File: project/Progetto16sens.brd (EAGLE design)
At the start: 228.6 x 231.1 mm, 148 parts, among them IC1 LMZ14202TZE-ADJ_NOPB, J2 455-1750-1-ND, M1 43650-0201, M2 43650-0201, M3 43650-0201, M4 43650-0201, M5 ARDUINO-PRO-MINI, SW1 TL32PO, SW2 TL32PO, SW3 TL32PO

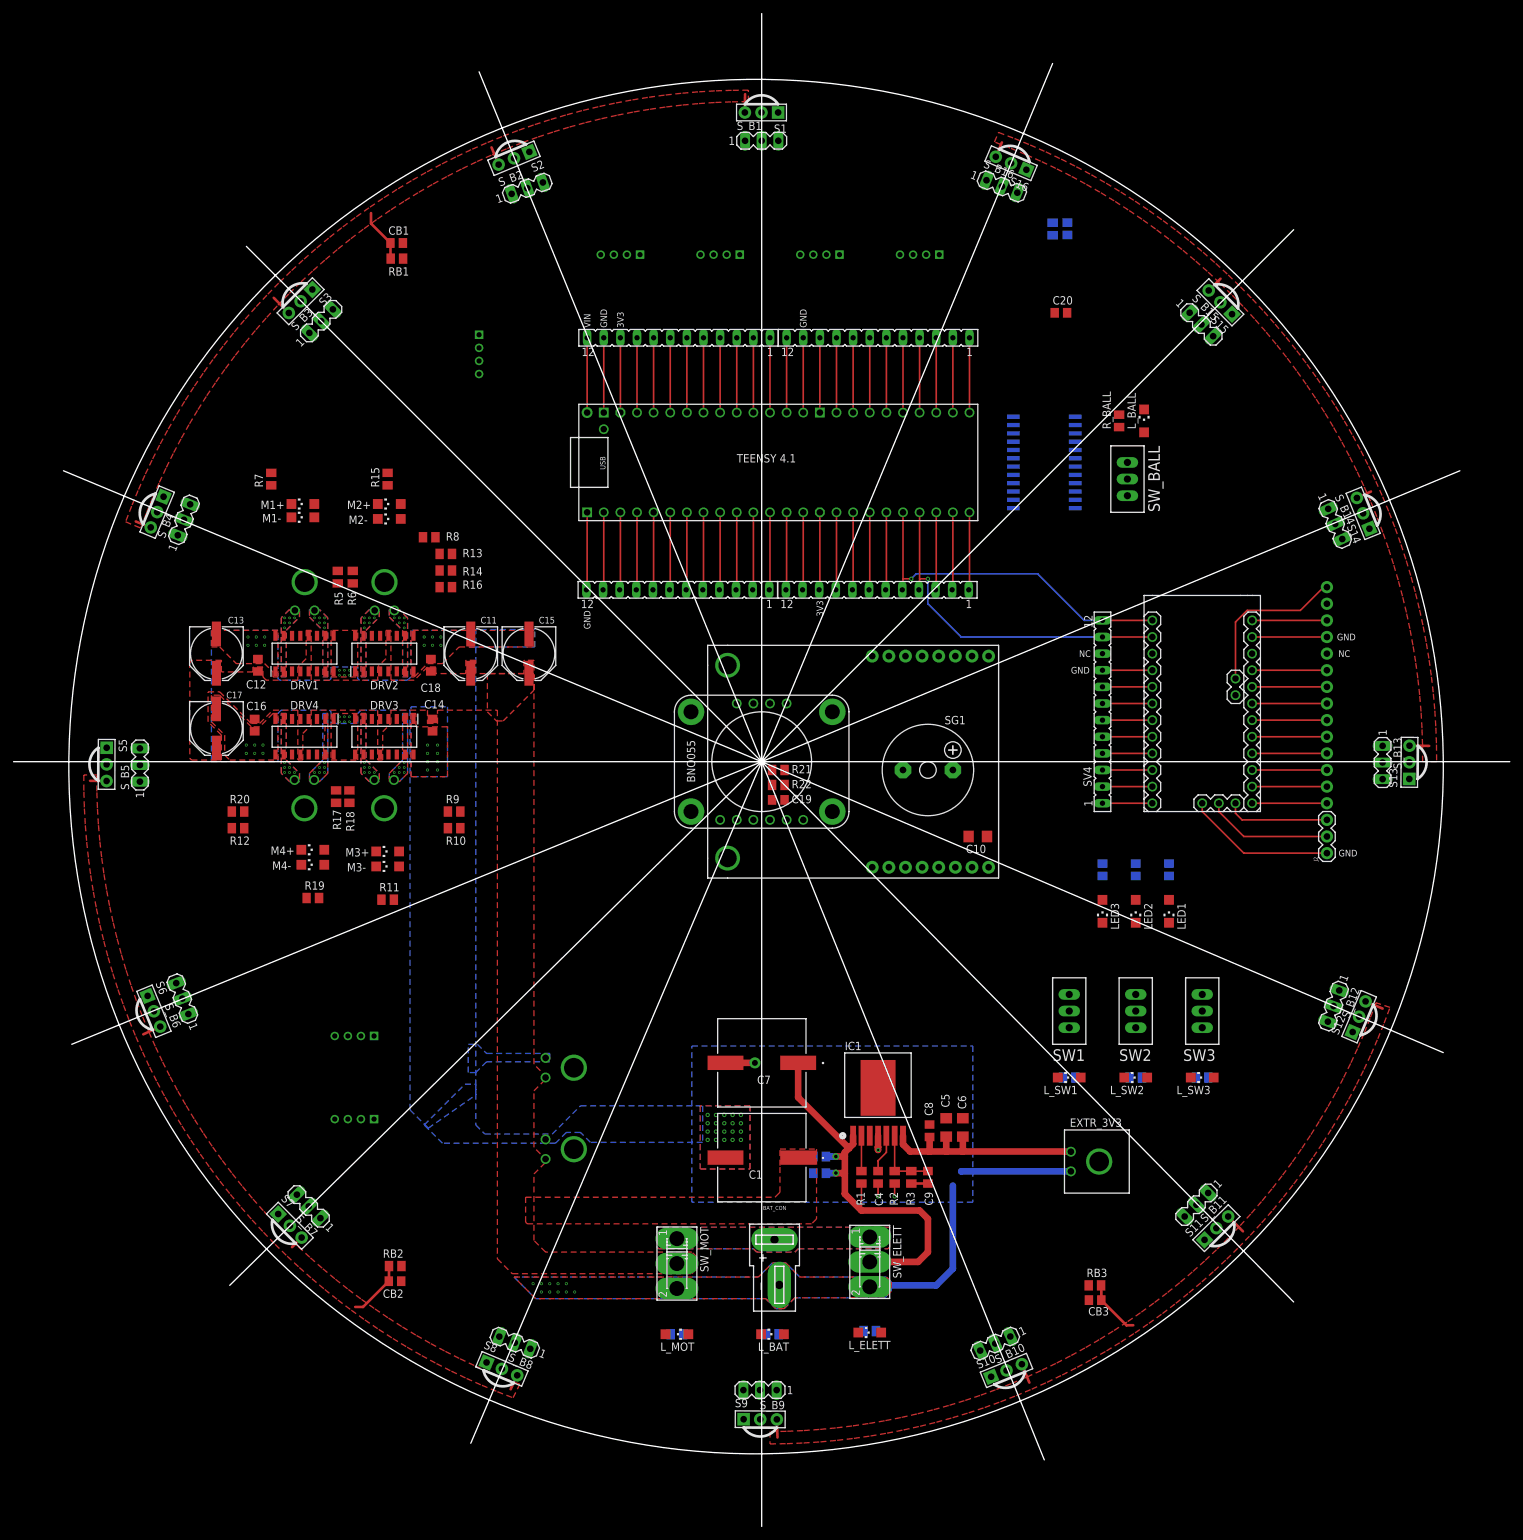
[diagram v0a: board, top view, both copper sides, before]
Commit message: continuing brd
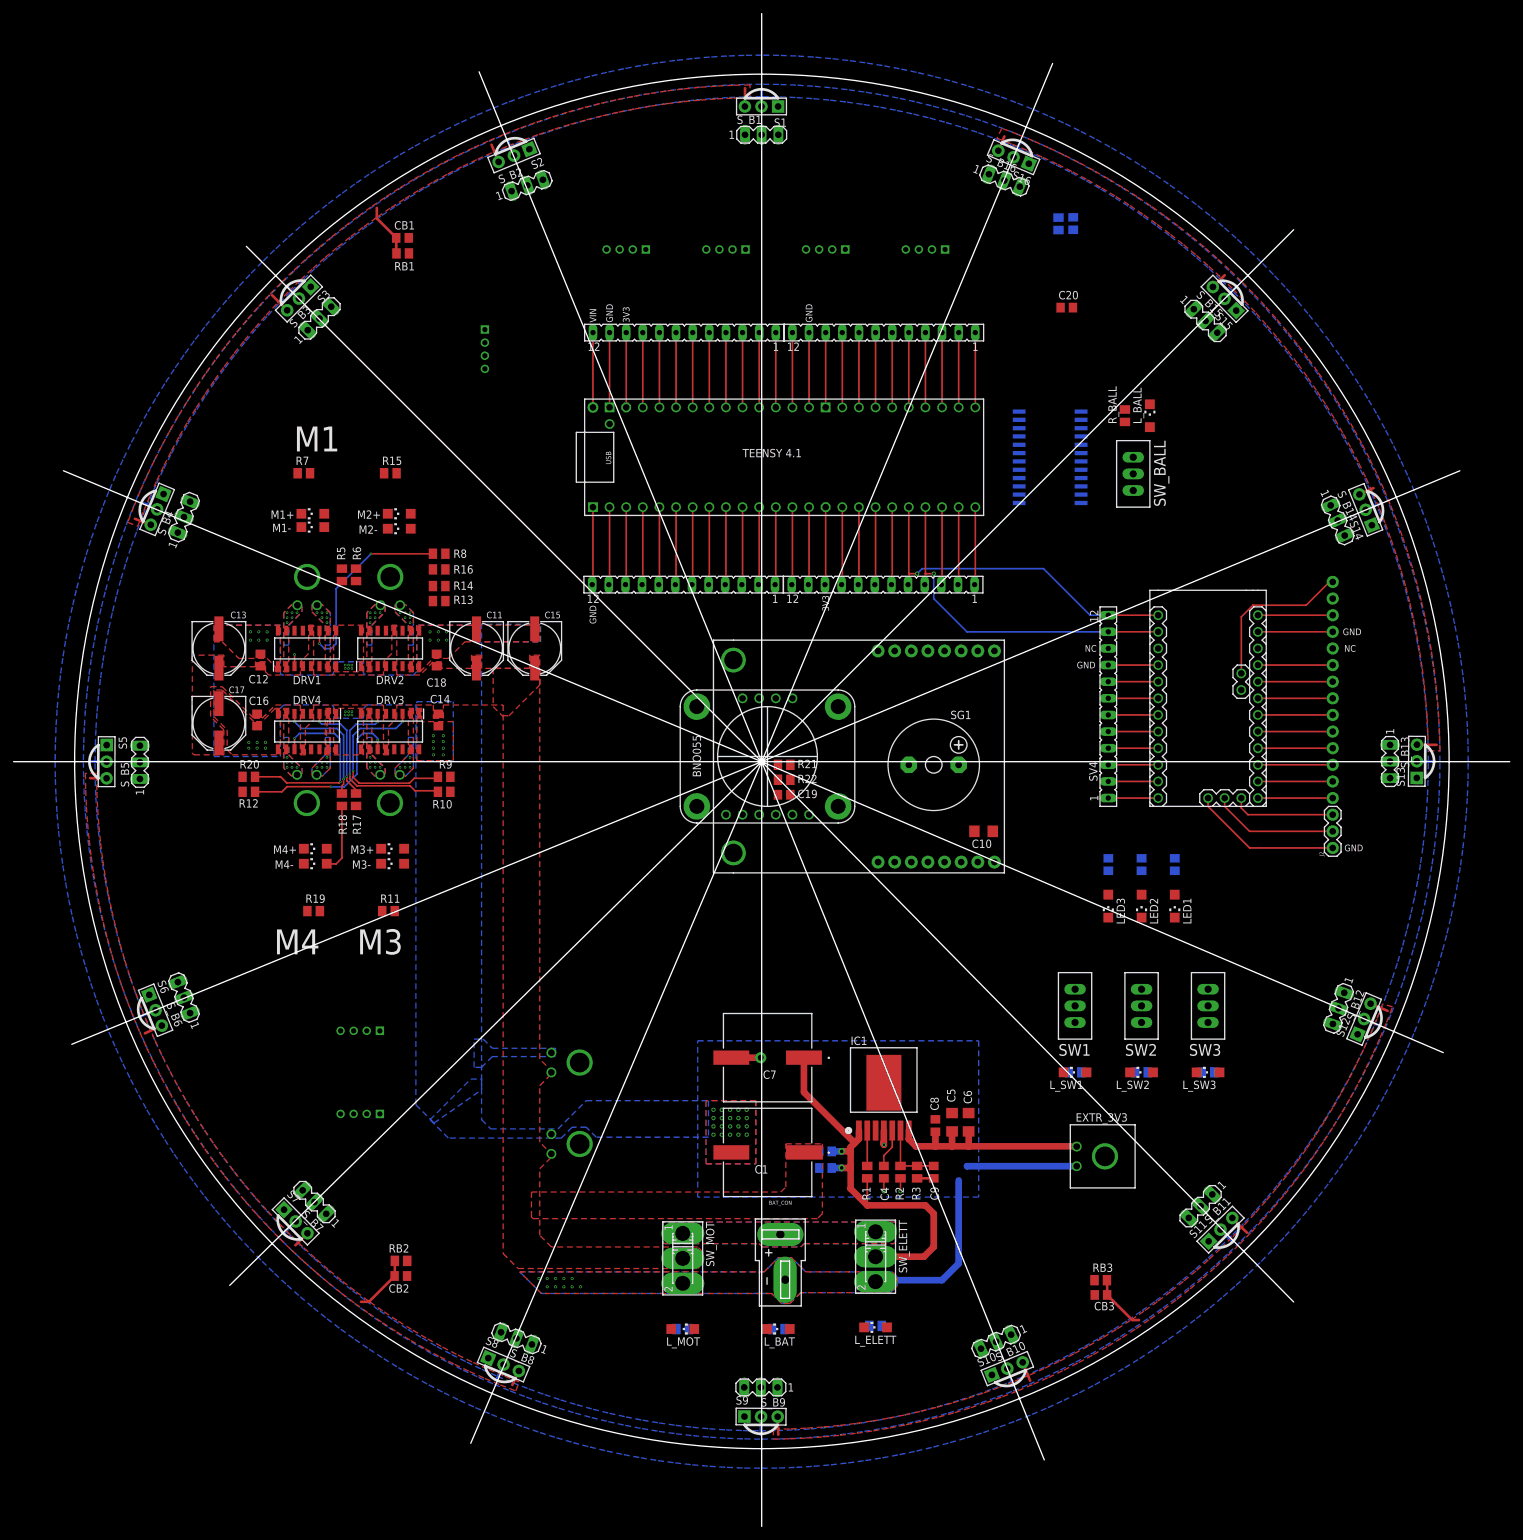
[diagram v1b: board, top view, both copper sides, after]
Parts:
- moved R13 7.28 mm to (-49.3, 24.5), turned to 180 degrees
- moved R12 5.80 mm to (-78.4, -4.60), turned to 180 degrees
- moved R10 5.76 mm to (-48.5, -4.60), turned to 180 degrees
- moved R20 5.56 mm to (-78.4, -2.31), turned to 180 degrees
- moved R9 5.52 mm to (-48.5, -2.31), turned to 180 degrees
- moved R7 5.06 mm to (-69.9, 44.1), turned to 0 degrees
- moved R17 3.09 mm to (-62.0, -5.81)
- moved R8 2.94 mm to (-49.3, 31.8)
- moved R16 2.88 mm to (-49.3, 29.4)
- moved R14 2.59 mm to (-49.3, 26.8), turned to 180 degrees
- moved M2- 2.13 mm to (-55.4, 35.6)
- moved M1+ 2.13 mm to (-68.6, 37.9)
- moved M1- 2.13 mm to (-68.6, 35.8)
- moved M2+ 2.13 mm to (-55.4, 37.9)
- moved R19 2.01 mm to (-68.5, -22.8)
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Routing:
- net GND: track 130.8 -> 172.9 mm
- net N$24: track 0.00 -> 30.6 mm, vias 0 -> 2
- net N$25: track 0.00 -> 29.7 mm, vias 0 -> 2
- net N$36: track 0.00 -> 29.3 mm, vias 0 -> 2
- net N$26: track 0.00 -> 27.7 mm, vias 0 -> 2
- net N$28: track 0.00 -> 27.6 mm, vias 0 -> 2
- net N$34: track 0.00 -> 18.6 mm, vias 0 -> 2
- net N$33: track 0.00 -> 16.2 mm, vias 0 -> 2
- net M4_INB: track 11.9 -> 22.5 mm
- net N$22: track 0.00 -> 1.79 mm, vias 0 -> 1
- net PWR_B2: track 18.9 -> 19.4 mm
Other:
- outline, holes or cut-outs redrawn
